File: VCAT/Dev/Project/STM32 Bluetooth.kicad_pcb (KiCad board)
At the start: 4 copper layers, 49.5 x 47.5 mm, 41 parts, among them J1 USB_C_Receptacle_USB2.0_16P, J2 Conn_ARM_SWD_TagConnect_TC2030, J3 Conn_01x04, J4 Conn_Coaxial, SW1 SW_Push, U1 MIC5365-3.3YD5, U2 USBLC6-2SC6, U3 STM32WB55CEUx, Y1 32Khz768, Y2 32Mhz

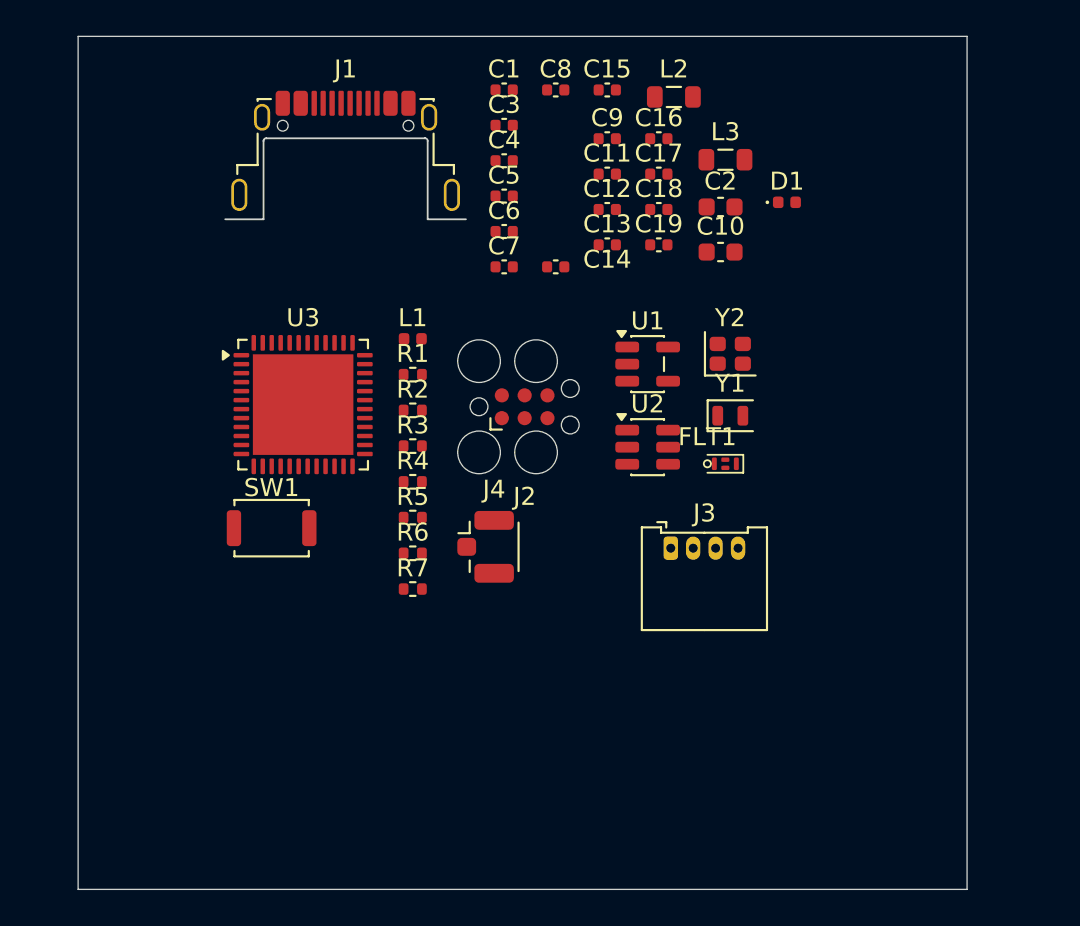
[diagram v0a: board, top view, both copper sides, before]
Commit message: 1.5
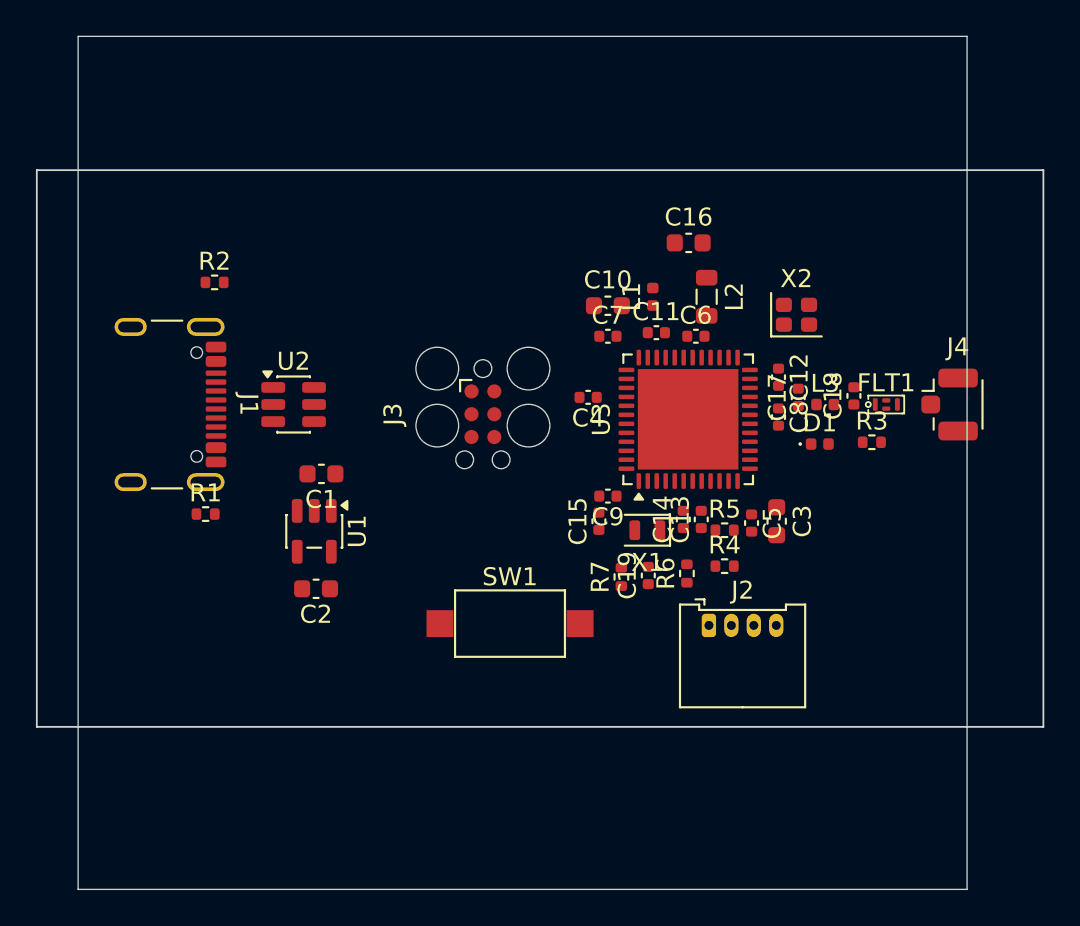
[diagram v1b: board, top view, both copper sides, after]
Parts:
- removed Y1: 32Khz768, Crystal:Crystal_SMD_2012-2Pin_2.0x1.2mm
- removed Y2: 32Mhz, Crystal:Crystal_SMD_2016-4Pin_2.0x1.6mm
- added X1: 32kHz768, Crystal:Crystal_SMD_2012-2Pin_2.0x1.2mm, F.Cu at (98.7, 87.0)
- added X2: 32MHz, Crystal:Crystal_SMD_2016-4Pin_2.0x1.6mm, F.Cu at (107.0, 75.0)
- C1, C16, C3: value 100n -> 4u7; footprint Capacitor_SMD:C_0402_1005Metric -> Capacitor_SMD:C_0603_1608Metric
- C13: value C -> 100n
- C14: value 100n -> 10p
- C15: value C -> 10p
- C17: value 100n -> 0p8
- C18: value 0p8 -> 0p3
- C19: value 0p3 -> 100n
- FLT1: footprint layout:DLF162500LT-5028A1 -> Library:DLF162500LT-5028A1
- J1: value USB_C_Receptacle_USB2.0_16P -> USB_C_Receptacle_USB2.0; footprint Connector_USB:USB_C_Receptacle_Amphenol_12401948E412A -> Connector_USB:USB_C_Receptacle_GCT_USB4105-xx-A_16P_TopMnt_Horizontal
- J2: value Conn_ARM_SWD_TagConnect_TC2030 -> Conn_01x04; footprint Connector:Tag-Connect_TC2030-IDC-FP_2x03_P1.27mm_Vertical -> Connector_Molex:Molex_PicoBlade_53048-0410_1x04_P1.25mm_Horizontal
- J3: value Conn_01x04 -> TC2030; footprint Connector_Molex:Molex_PicoBlade_53048-0410_1x04_P1.25mm_Horizontal -> Connector:Tag-Connect_TC2030-IDC-FP_2x03_P1.27mm_Vertical
- L3: value 10u -> 2n7; footprint Inductor_SMD:L_0805_2012Metric -> Inductor_SMD:L_0402_1005Metric
- SW1: footprint Button_Switch_SMD:SW_Push_SPST_NO_Alps_SKRK -> Button_Switch_SMD:SW_SPST_CK_RS282G05A3
- U1: footprint Package_TO_SOT_SMD:TSOT-23-5 -> Package_TO_SOT_SMD:SOT-23-5
- U3: value STM32WB55CEUx -> STM32WB55CEU
- moved C2 31.0 mm to (80.2, 90.3), turned to 180 degrees
- moved J4 27.0 mm to (116.0, 80.0)
- moved C3 26.8 mm to (105.9, 86.5), turned to -90 degrees
- moved R3 25.6 mm to (111.2, 82.1)
- moved C15 24.0 mm to (96.0, 86.5), turned to 90 degrees
- moved C1 23.7 mm to (80.5, 83.9), turned to 180 degrees
- moved C5 22.8 mm to (104.5, 86.6), turned to -90 degrees
- moved C8 22.0 mm to (106.0, 80.7), turned to -90 degrees
- moved U3 21.5 mm to (101.0, 80.8), turned to 90 degrees
- moved U1 20.8 mm to (80.2, 87.1), turned to -90 degrees
- moved C9 19.9 mm to (96.5, 85.1), turned to 180 degrees
- moved U2 19.9 mm to (79.0, 80.0)
- moved C19 18.4 mm to (98.8, 89.5), turned to 90 degrees
- moved R4 18.0 mm to (103.0, 89.0)
- moved R5 17.4 mm to (103.0, 87.0)
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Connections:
- net +3.3V renamed +3V3
- net /<NO NET> renamed /USB_D-
- net /LEDA renamed Net-(D1-A)
- net /LEDC renamed Net-(D1-K)
- net /LSE_in renamed /LSE_IN
- net Net-(FLT1-OUT) renamed /RF_ANT
- C13 pad 1: /LSE_out -> /SWD_NRST
- C14 pad 1: Net-(J2-~{RESET}) -> /LSE_OUT
- C17 pad 1: /BOOT0 -> /RF
- C18 pad 1: /RF -> /RF_MATCH
- C19 pad 1: Net-(FLT1-IN) -> /BOOT0
- FLT1 pad 1: Net-(FLT1-IN) -> /RF_MATCH
- J1 pad SH: GND -> (no net)
- J2 pad 2: /SVD_DIO -> /UART_TXC
- J2 pad 3: Net-(J2-~{RESET}) -> /UART_RXC
- J2 pad 4: /SVD_CLK -> GND
- J3 pad 2: Net-(J3-Pin_2) -> /SWD_DIO
- J3 pad 3: Net-(J3-Pin_3) -> /SWD_NRST
- J3 pad 4: GND -> /SWD_CLK
- L1 pad 2: /SMPSLX -> /SMPSLXL
- L2 pad 1: /SMPSLX -> /SMPSLXL
- L3 pad 2: Net-(FLT1-IN) -> /RF_MATCH
- R1 pad 1: GND -> Net-(J1-CC2)
- R1 pad 2: Net-(J1-CC2) -> GND
- R2 pad 1: GND -> Net-(J1-CC1)
- R2 pad 2: Net-(J1-CC1) -> GND
- R4 pad 1: Net-(J3-Pin_2) -> /UART_TXC
- R5 pad 1: Net-(J3-Pin_3) -> /UART_RXC
- U3 pad 24: /HSE_out -> /HCE_OUT
- U3 pad 25: /HSE_in -> /HCE_IN
- U3 pad 3: /LSE_out -> /LSE_OUT
- U3 pad 39: /SVD_DIO -> /SWD_DIO
- U3 pad 41: /SVD_CLK -> /SWD_CLK
- U3 pad 43: /SVD_TRC -> /SWD_TRC
- U3 pad 7: Net-(J2-~{RESET}) -> /SWD_NRST
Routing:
- added copper zone on In1.Cu, net GND
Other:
- board size 49.5 x 47.5 mm -> 56 x 47.5 mm
